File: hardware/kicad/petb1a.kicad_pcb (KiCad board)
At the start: 4 copper layers, 39.6 x 61 mm, 48 parts, among them J1 TYPEC-304-ACP16, J2 EXP1, J3 EXP2, J4 Qwiic, SW1 TD-1183SA-1.5H-250, SW2 TD-1183SA-1.5H-250, U1 USBLC6-2P6, U2 ESP32-S3-WROOM-1, U3 XC6220B331MR-G, U4 BME680

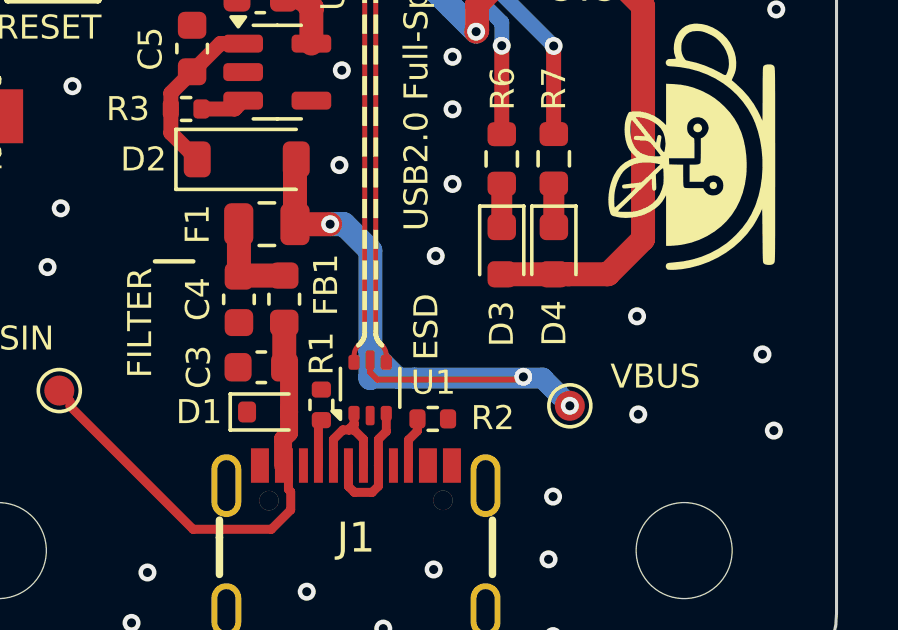
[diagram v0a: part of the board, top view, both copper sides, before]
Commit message: update pcb
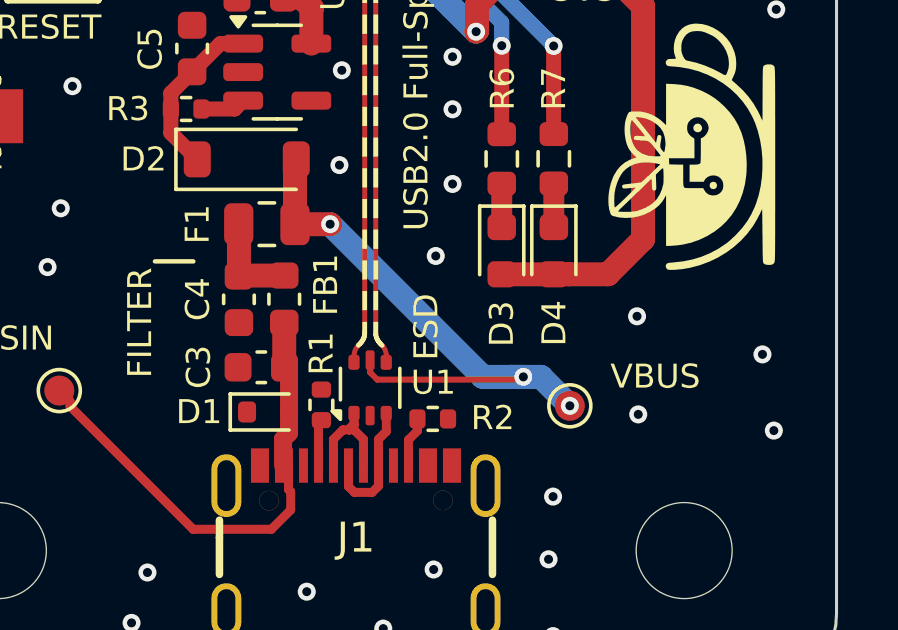
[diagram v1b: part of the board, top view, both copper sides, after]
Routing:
- net VBUS: track 23.4 -> 20.0 mm
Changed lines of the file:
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@@
 	)
 	(segment
-		(start 148.22 103.42)
-		(end 148.68 103.42)
+		(start 155.246 108.51)
+		(end 156.21 109.474)
 		(width 0.8)
 		(layer "B.Cu")
@@
 	)
 	(segment
-		(start 149.56 104.3)
-		(end 149.56 107.61)
+		(start 154.22 108.51)
+		(end 155.246 108.51)
 		(width 0.8)
 		(layer "B.Cu")
@@
 	)
 	(segment
-		(start 149.56 108.545196)
-		(end 149.555205 108.549991)
+		(start 154.22 108.51)
+		(end 154.66 108.51)
 		(width 0.8)
 		(layer "B.Cu")
@@
 	)
 	(segment
-		(start 150.49 108.549991)
-		(end 149.555205 108.549991)
-		(width 0.7)
+		(start 148.22 103.42)
+		(end 153.31 108.51)
+		(width 0.8)
 		(layer "B.Cu")
 		(net 8)
@@
 		(start 156.216 109.474)
 		(end 156.21 109.474)
-		(width 0.7)
-		(layer "B.Cu")
-		(net 8)
-	)
-	(segment
-		(start 155.299991 108.549991)
-		(end 151.03 108.549991)
-		(width 0.7)
-		(layer "B.Cu")
-		(net 8)
-	)
-	(segment
-		(start 151.03 108.549991)
-		(end 150.49 108.549991)
-		(width 0.7)
-		(layer "B.Cu")
-		(net 8)
-	)
-	(segment
-		(start 148.68 103.42)
-		(end 149.56 104.3)
-		(width 0.8)
-		(layer "B.Cu")
-		(net 8)
-	)
-	(segment
-		(start 150.49 108.549991)
-		(end 150.49 108.54)
 		(width 0.7)
 		(layer "B.Cu")
@@
 	)
 	(segment
-		(start 149.56 107.61)
-		(end 149.56 108.545196)
+		(start 153.31 108.51)
+		(end 154.22 108.51)
 		(width 0.8)
 		(layer "B.Cu")
 		(net 8)
-	)
-	(segment
-		(start 150.49 108.54)
-		(end 149.56 107.61)
-		(width 0.7)
-		(layer "B.Cu")
-		(net 8)
-	)
-	(segment
-		(start 156.22 109.47)
-		(end 155.299991 108.549991)
-		(width 0.7)
-		(layer "B.Cu")
-		(net 8)
